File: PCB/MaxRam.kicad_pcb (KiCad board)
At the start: 2 copper layers, 74.9 x 40.6 mm, 15 parts, among them J1 CONN_01X14, J2 CONN_01X04, J3 CONN_02X05, J4 CONN_01X03, J5 CONN_01X03, J6 CONN_01X14, J7 CONN_01X02, U1 AS6C4008-55SIN, U2 SST39SF040, U3 ATF1502PLCC44, U4 DS1210

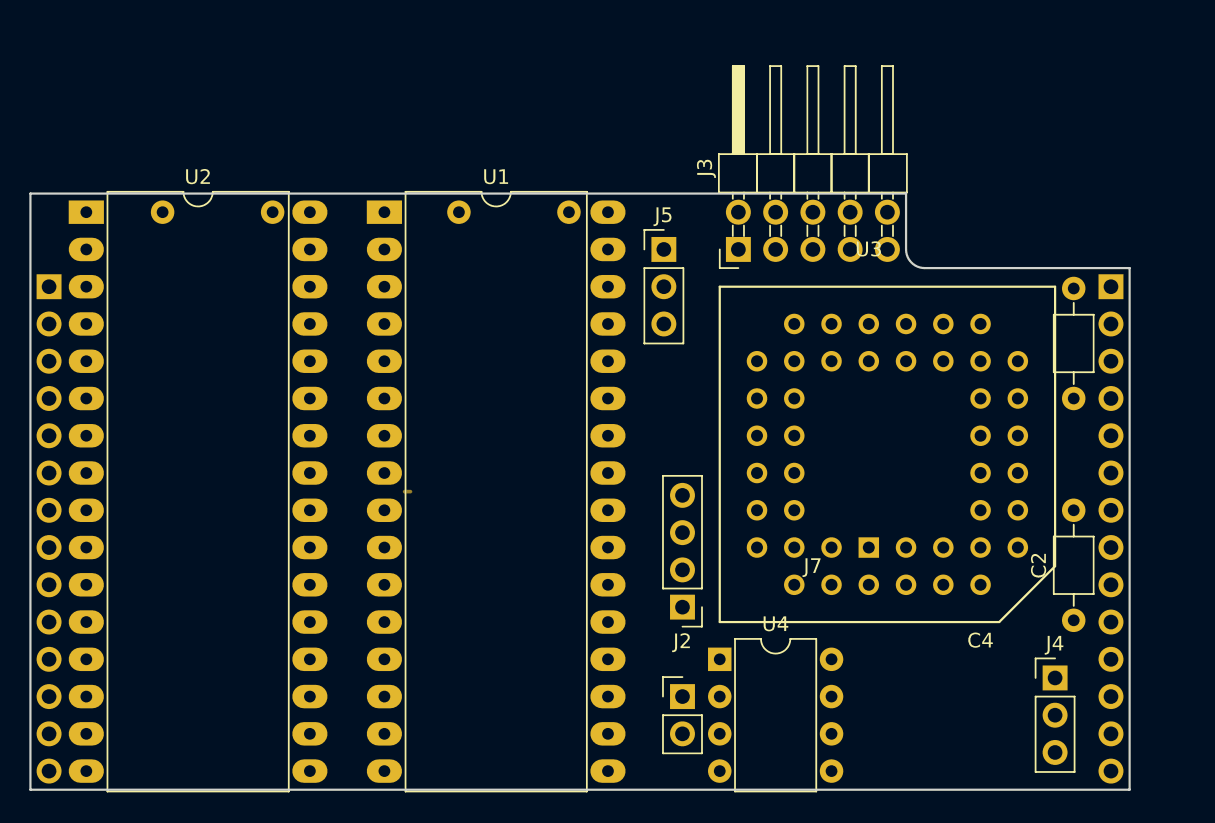
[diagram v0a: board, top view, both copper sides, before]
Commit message: Update PCB Still getting used to KiCad / PCB Design
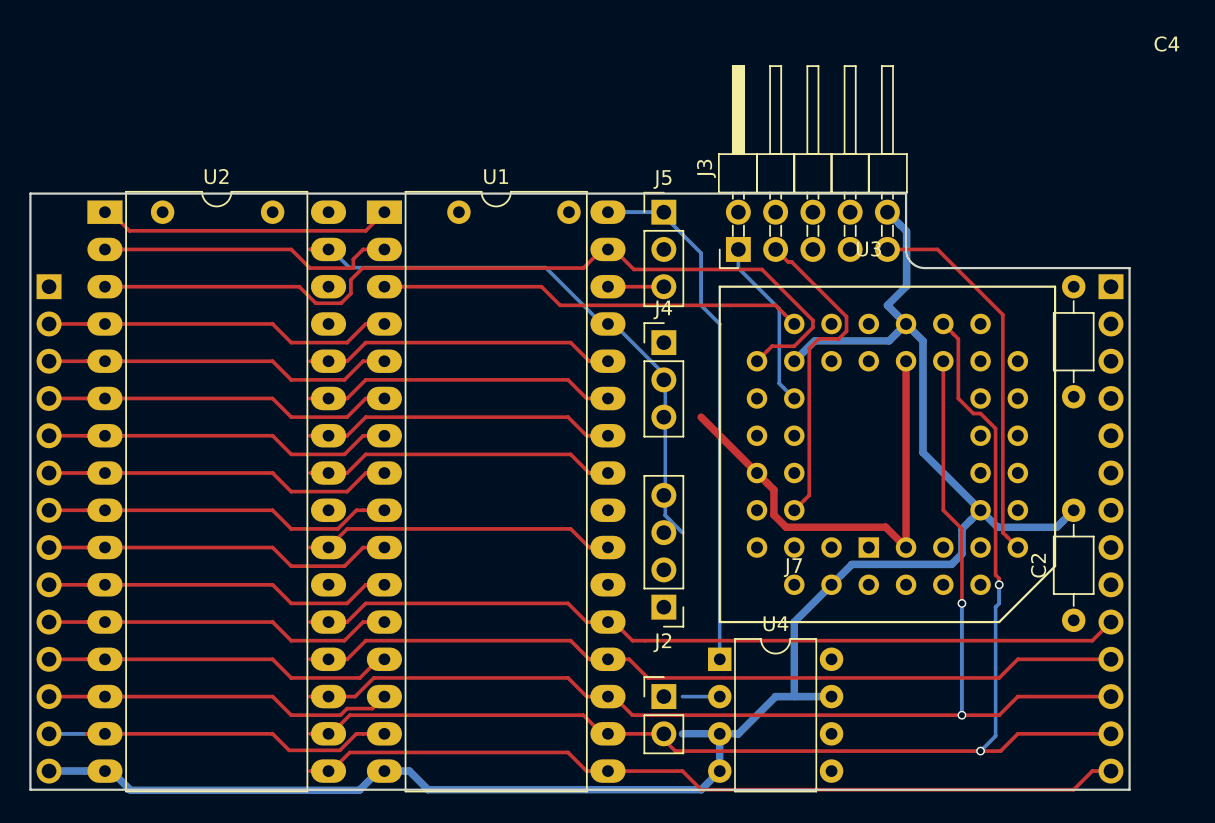
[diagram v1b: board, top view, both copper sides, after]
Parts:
- moved J4 35.1 mm to (153.7, 110.5)
- moved C4 7.62 mm to (181.6, 106.7), turned to 270 degrees
- moved C1 7.50 mm to (127.0, 101.6), turned to 180 degrees
- moved C3 7.50 mm to (147.2, 101.6), turned to 180 degrees
- moved J5 2.54 mm to (153.7, 101.6)
- moved J2 1.27 mm to (153.7, 128.5)
- moved J7 1.27 mm to (153.7, 134.6)
- moved U2 1.27 mm to (115.6, 101.6)
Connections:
- C1 pad 1: +5V -> Net-(C1-Pad1)
- C1 pad 2: Net-(C1-Pad2) -> GND
- C2 pad 2: Net-(C1-Pad2) -> GND
- C3 pad 2: Net-(C1-Pad2) -> GND
- C4 pad 2: Net-(C1-Pad2) -> GND
- J1 pad 14: Net-(C1-Pad2) -> GND
- J3 pad 10: Net-(C1-Pad2) -> GND
- J3 pad 2: Net-(C1-Pad2) -> GND
- J4 pad 1: Net-(J4-Pad1) -> /We
- J5 pad 2: /S18 -> /PIN30
- J6 pad 1: Net-(J6-Pad1) -> +5V
- J7 pad 2: Net-(C1-Pad2) -> GND
- U1 pad 16: Net-(C1-Pad2) -> GND
- U1 pad 24: /Romsel -> Net-(J6-Pad7)
- U1 pad 29: Net-(J4-Pad1) -> /We
- U1 pad 32: Net-(U1-Pad32) -> Net-(C1-Pad1)
- U2 pad 24: /Romsel -> Net-(J6-Pad7)
- U2 pad 30: /S18 -> /PIN30
- U2 pad 31: Net-(J4-Pad1) -> /We
- U3 pad 10: Net-(C1-Pad2) -> GND
- U3 pad 2: /Romsel -> Net-(J6-Pad7)
- U3 pad 22: Net-(C1-Pad2) -> GND
- U3 pad 30: Net-(C1-Pad2) -> GND
- U3 pad 40: Net-(U2-Pad22) -> Net-(U3-Pad40)
- U3 pad 42: Net-(C1-Pad2) -> GND
- U3 pad 44: /We -> /Romsel
- U4 pad 1: Net-(U1-Pad32) -> Net-(C1-Pad1)
- U4 pad 3: Net-(C1-Pad2) -> GND
- U4 pad 7: Net-(C1-Pad2) -> GND
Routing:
- net GND: track 0.00 -> 125.2 mm
- net /D4: track 0.00 -> 86.5 mm, vias 0 -> 2
- net /D5: track 0.00 -> 81.4 mm, vias 0 -> 2
- net /S15: track 0.00 -> 58.0 mm
- net /D3: track 0.00 -> 56.7 mm
- net /D7: track 0.00 -> 56.7 mm
- net /D6: track 0.00 -> 56.7 mm
- net +5V: track 0.00 -> 42.8 mm
- net /We: track 0.00 -> 29.1 mm
- net /S14: track 0.00 -> 29.0 mm
- net /TDI: track 0.00 -> 26.0 mm
- net Net-(C1-Pad1): track 0.00 -> 24.3 mm
- net /D1: track 0.00 -> 23.9 mm
- net /A0: track 0.00 -> 23.9 mm
- net /A4: track 0.00 -> 23.9 mm
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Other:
- net class Power added: clearance 0.2, trace_width 0.508, via_dia 0.6, via_drill 0.4
